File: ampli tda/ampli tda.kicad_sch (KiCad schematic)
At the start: 19 parts, among them J1 Barrel_Jack, J2 Conn_01x03_Pin, U1 TDA2003

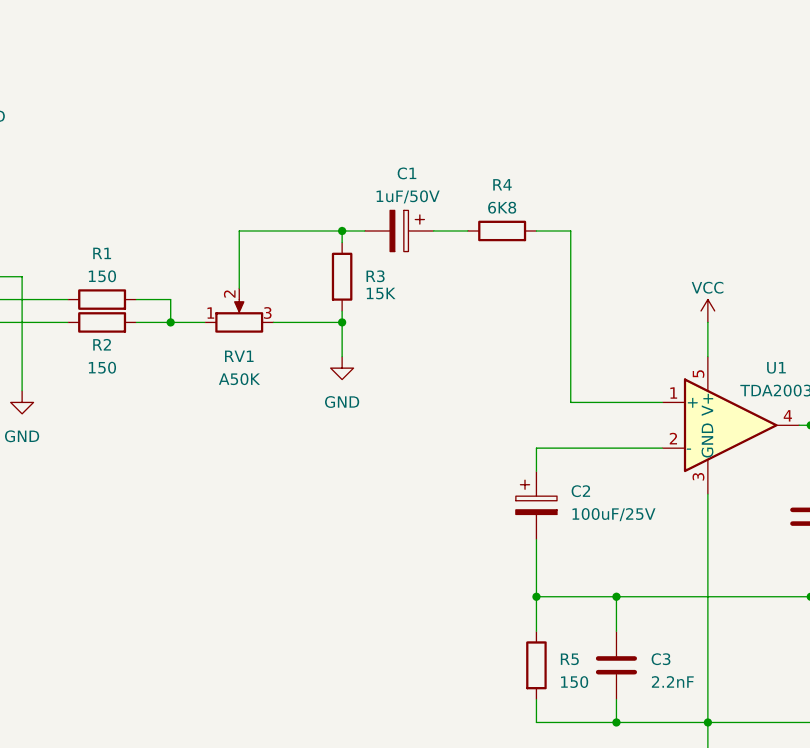
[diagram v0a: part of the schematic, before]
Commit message: REV 0.2
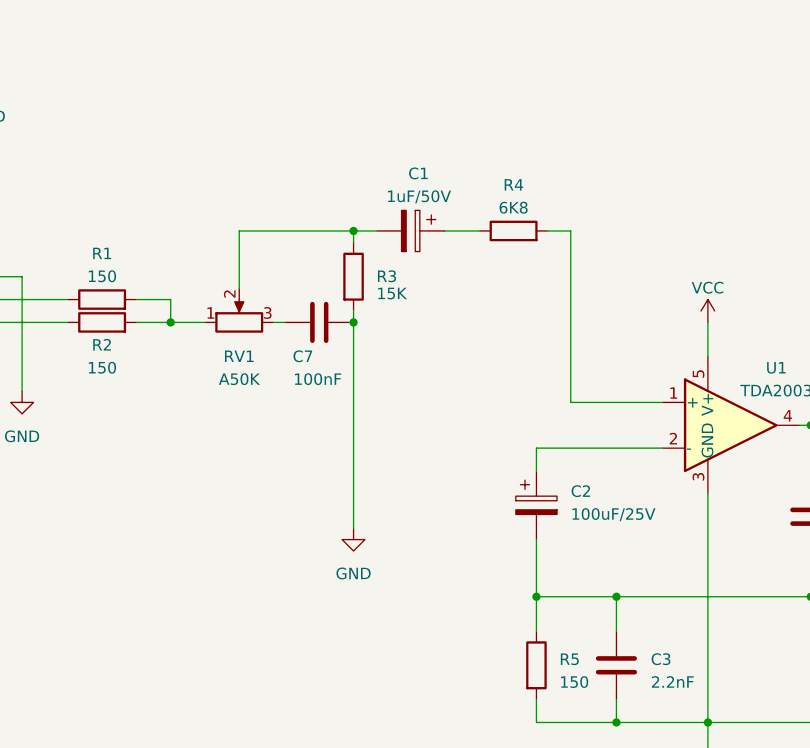
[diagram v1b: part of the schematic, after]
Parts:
- added C7: 100nF, Capacitor_THT:C_Disc_D7.5mm_W2.5mm_P5.00mm, symbol Device:C
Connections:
- net GND: now also C7.2; no longer RV1.3
- new net: C7.1, RV1.3
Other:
- moved on the sheet: C1, R3, R4
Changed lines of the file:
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@@
   (junction (at 144.78 114.3) (diameter 0) (color 0 0 0 0)
   )
-  (junction (at 104.14 59.69) (diameter 0) (color 0 0 0 0)
+  (junction (at 105.41 59.69) (diameter 0) (color 0 0 0 0)
   )
   (junction (at 181.61 114.3) (diameter 0) (color 0 0 0 0)
@@
   (junction (at 156.21 81.28) (diameter 0) (color 0 0 0 0)
   )
-  (junction (at 104.14 69.85) (diameter 0) (color 0 0 0 0)
-  )
   (junction (at 181.61 81.28) (diameter 0) (color 0 0 0 0)
   )
@@
   (junction (at 125.73 100.33) (diameter 0) (color 0 0 0 0)
   )
-  (wire (pts (xy 104.14 59.69) (xy 104.14 60.96))
+  (junction (at 105.41 69.85) (diameter 0) (color 0 0 0 0)
+  )
+  (wire (pts (xy 105.41 59.69) (xy 105.41 60.96))
     (stroke (width 0) (type default))
   )
@@
     (stroke (width 0) (type default))
   )
-  (wire (pts (xy 104.14 69.85) (xy 104.14 68.58))
-    (stroke (width 0) (type default))
-  )
-  (wire (pts (xy 114.3 59.69) (xy 118.11 59.69))
+  (wire (pts (xy 115.57 59.69) (xy 119.38 59.69))
     (stroke (width 0) (type default))
   )
@@
     (stroke (width 0) (type default))
   )
+  (wire (pts (xy 97.79 69.85) (xy 96.52 69.85))
+    (stroke (width 0) (type default))
+  )
   (wire (pts (xy 92.71 59.69) (xy 92.71 66.04))
     (stroke (width 0) (type default))
   )
-  (wire (pts (xy 92.71 59.69) (xy 104.14 59.69))
+  (wire (pts (xy 92.71 59.69) (xy 105.41 59.69))
     (stroke (width 0) (type default))
   )
@@
     (stroke (width 0) (type default))
   )
+  (wire (pts (xy 105.41 69.85) (xy 105.41 92.71))
+    (stroke (width 0) (type default))
+  )
   (wire (pts (xy 125.73 104.14) (xy 125.73 100.33))
     (stroke (width 0) (type default))
@@
     (stroke (width 0) (type default))
   )
-  (wire (pts (xy 104.14 69.85) (xy 104.14 73.66))
-    (stroke (width 0) (type default))
-  )
-  (wire (pts (xy 104.14 59.69) (xy 106.68 59.69))
+  (wire (pts (xy 105.41 68.58) (xy 105.41 69.85))
+    (stroke (width 0) (type default))
+  )
+  (wire (pts (xy 105.41 59.69) (xy 107.95 59.69))
     (stroke (width 0) (type default))
   )
@@
     (stroke (width 0) (type default))
   )
-  (wire (pts (xy 96.52 69.85) (xy 104.14 69.85))
-    (stroke (width 0) (type default))
-  )
-  (wire (pts (xy 125.73 59.69) (xy 129.54 59.69))
+  (wire (pts (xy 127 59.69) (xy 129.54 59.69))
     (stroke (width 0) (type default))
   )
@@
     )
   )
-  (symbol (lib_id "Device:R") (at 121.92 59.69 90) (unit 1)
-    (in_bom yes) (on_board yes) (dnp no) (fields_autoplaced)
-    (property "Reference" "R4" (at 121.92 54.61 90)
-      (effects (font (size 1.27 1.27)))
-    )
-    (property "Value" "6K8" (at 121.92 57.15 90)
-      (effects (font (size 1.27 1.27)))
-    )
-    (property "Footprint" "Resistor_THT:R_Axial_DIN0207_L6.3mm_D2.5mm_P7.62mm_Horizontal" (at 121.92 61.468 90)
-      (effects (font (size 1.27 1.27)) hide)
-    )
-    (property "Datasheet" "~" (at 121.92 59.69 0)
+  (symbol (lib_id "Device:R") (at 123.19 59.69 90) (unit 1)
+    (in_bom yes) (on_board yes) (dnp no) (fields_autoplaced)
+    (property "Reference" "R4" (at 123.19 54.61 90)
+      (effects (font (size 1.27 1.27)))
+    )
+    (property "Value" "6K8" (at 123.19 57.15 90)
+      (effects (font (size 1.27 1.27)))
+    )
+    (property "Footprint" "Resistor_THT:R_Axial_DIN0207_L6.3mm_D2.5mm_P7.62mm_Horizontal" (at 123.19 61.468 90)
+      (effects (font (size 1.27 1.27)) hide)
+    )
+    (property "Datasheet" "~" (at 123.19 59.69 0)
       (effects (font (size 1.27 1.27)) hide)
     )
@@
     )
   )
-  (symbol (lib_id "power:GND") (at 104.14 73.66 0) (unit 1)
-    (in_bom yes) (on_board yes) (dnp no) (fields_autoplaced)
-    (property "Reference" "#PWR04" (at 104.14 80.01 0)
-      (effects (font (size 1.27 1.27)) hide)
-    )
-    (property "Value" "GND" (at 104.14 78.74 0)
-      (effects (font (size 1.27 1.27)))
-    )
-    (property "Footprint" "" (at 104.14 73.66 0)
-      (effects (font (size 1.27 1.27)) hide)
-    )
-    (property "Datasheet" "" (at 104.14 73.66 0)
+  (symbol (lib_id "power:GND") (at 105.41 92.71 0) (unit 1)
+    (in_bom yes) (on_board yes) (dnp no) (fields_autoplaced)
+    (property "Reference" "#PWR04" (at 105.41 99.06 0)
+      (effects (font (size 1.27 1.27)) hide)
+    )
+    (property "Value" "GND" (at 105.41 97.79 0)
+      (effects (font (size 1.27 1.27)))
+    )
+    (property "Footprint" "" (at 105.41 92.71 0)
+      (effects (font (size 1.27 1.27)) hide)
+    )
+    (property "Datasheet" "" (at 105.41 92.71 0)
       (effects (font (size 1.27 1.27)) hide)
     )
@@
     )
   )
+  (symbol (lib_id "Device:C") (at 101.6 69.85 90) (mirror x) (unit 1)
+    (in_bom yes) (on_board yes) (dnp no)
+    (property "Reference" "C7" (at 100.965 73.66 90)
+      (effects (font (size 1.27 1.27)) (justify left))
+    )
+    (property "Value" "100nF" (at 104.14 76.2 90)
+      (effects (font (size 1.27 1.27)) (justify left))
+    )
+    (property "Footprint" "Capacitor_THT:C_Disc_D7.5mm_W2.5mm_P5.00mm" (at 105.41 70.8152 0)
+      (effects (font (size 1.27 1.27)) hide)
+    )
+    (property "Datasheet" "~" (at 101.6 69.85 0)
+      (effects (font (size 1.27 1.27)) hide)
+    )
+    (pin "1")
+    (pin "2")
+    (instances
+      (project "ampli tda"
+        (path "/6bb2531f-dc70-427d-8480-c768664d9409"
+          (reference "C7") (unit 1)
+        )
+      )
+    )
+  )
   (symbol (lib_id "Device:Speaker") (at 201.93 81.28 0) (unit 1)
     (in_bom yes) (on_board yes) (dnp no) (fields_autoplaced)
@@
     )
   )
-  (symbol (lib_id "Device:R") (at 104.14 64.77 0) (unit 1)
+  (symbol (lib_id "Device:R") (at 105.41 64.77 0) (unit 1)
     (in_bom yes) (on_board yes) (dnp no)
-    (property "Reference" "R3" (at 106.68 64.77 0)
-      (effects (font (size 1.27 1.27)) (justify left))
-    )
-    (property "Value" "15K" (at 106.68 66.675 0)
-      (effects (font (size 1.27 1.27)) (justify left))
-    )
-    (property "Footprint" "Resistor_THT:R_Axial_DIN0207_L6.3mm_D2.5mm_P7.62mm_Horizontal" (at 102.362 64.77 90)
-      (effects (font (size 1.27 1.27)) hide)
-    )
-    (property "Datasheet" "~" (at 104.14 64.77 0)
+    (property "Reference" "R3" (at 107.95 64.77 0)
+      (effects (font (size 1.27 1.27)) (justify left))
+    )
+    (property "Value" "15K" (at 107.95 66.675 0)
+      (effects (font (size 1.27 1.27)) (justify left))
+    )
+    (property "Footprint" "Resistor_THT:R_Axial_DIN0207_L6.3mm_D2.5mm_P7.62mm_Horizontal" (at 103.632 64.77 90)
+      (effects (font (size 1.27 1.27)) hide)
+    )
+    (property "Datasheet" "~" (at 105.41 64.77 0)
       (effects (font (size 1.27 1.27)) hide)
     )
@@
     )
   )
-  (symbol (lib_id "Device:C_Polarized") (at 110.49 59.69 270) (unit 1)
-    (in_bom yes) (on_board yes) (dnp no) (fields_autoplaced)
-    (property "Reference" "C1" (at 111.379 53.34 90)
-      (effects (font (size 1.27 1.27)))
-    )
-    (property "Value" "1uF/50V" (at 111.379 55.88 90)
-      (effects (font (size 1.27 1.27)))
-    )
-    (property "Footprint" "Capacitor_THT:CP_Radial_D5.0mm_P2.50mm" (at 106.68 60.6552 0)
-      (effects (font (size 1.27 1.27)) hide)
-    )
-    (property "Datasheet" "~" (at 110.49 59.69 0)
-      (effects (font (size 1.27 1.27)) hide)
-    )
+  (symbol (lib_id "Device:C_Polarized") (at 111.76 59.69 270) (unit 1)
+    (in_bom yes) (on_board yes) (dnp no) (fields_autoplaced)
+    (property "Reference" "C1" (at 112.649 53.34 90)
+      (effects (font (size 1.27 1.27)))
+    )
+    (property "Value" "1uF/50V" (at 112.649 55.88 90)
+      (effects (font (size 1.27 1.27)))
+    )
+    (property "Footprint" "Capacitor_THT:CP_Radial_D5.0mm_P2.50mm" (at 107.95 60.6552 0)
+      (effects (font (size 1.27 1.27)) hide)
+    )
+    (property "Datasheet" "~" (at 111.76 59.69 0)
+      (effects (font (size 1.27 1.27)) hide)
+    )
